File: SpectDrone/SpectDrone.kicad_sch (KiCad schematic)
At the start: 139 parts, among them J1 Conn_02x03_Counter_Clockwise, J1-1 Conn_01x04_Male, J1-2 Conn_01x04_Male, J2 GPS, J3 Barrel_Jack, J3V1-1 Conn_01x01_Male, J3V3 Conn_01x01_Male, J4 BME280, J4V0-1 Conn_01x01_Male, J5 RFShield_OnePiece, J5-1 BNO055-1, J5-2 BNO055-2, J5V3-1 Conn_01x01_Male, J5V3-2 Conn_01x01_Male, J6 Conn_02x16_Counter_Clockwise, J7 Conn_02x16_Counter_Clockwise, Q1 FDN340P, Q2 FDN340P, SW0 SW_Push, SW1 SW_Push, SW10 SW_Push, SW2 SW_Push, SW3 SW_Push, SW4 SW_Push, SW5 SW_Push, SW6 SW_Push, SW7 SW_Push, SW8 SW_Push, SW9 SW_Push, U1 C12666MA, U10 TXS0102DCUR, U11 PCA9306DC, U12 AD799x, U2 C12666MA, U3 MCP112-450E/TO, U4 LM7805_SOT223, U5 MCP112-450E/TO, U6 LM7805_SOT223, U7 Teensy4.0

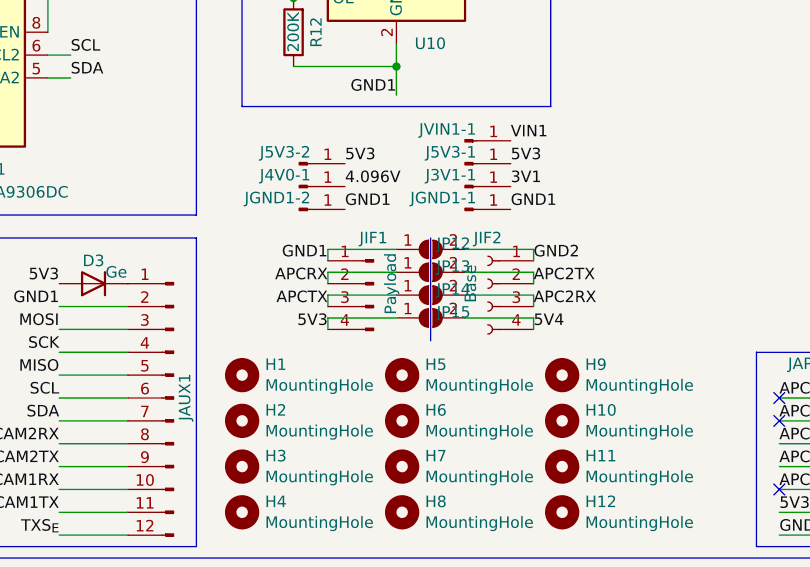
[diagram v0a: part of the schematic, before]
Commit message: SpectDrone Development
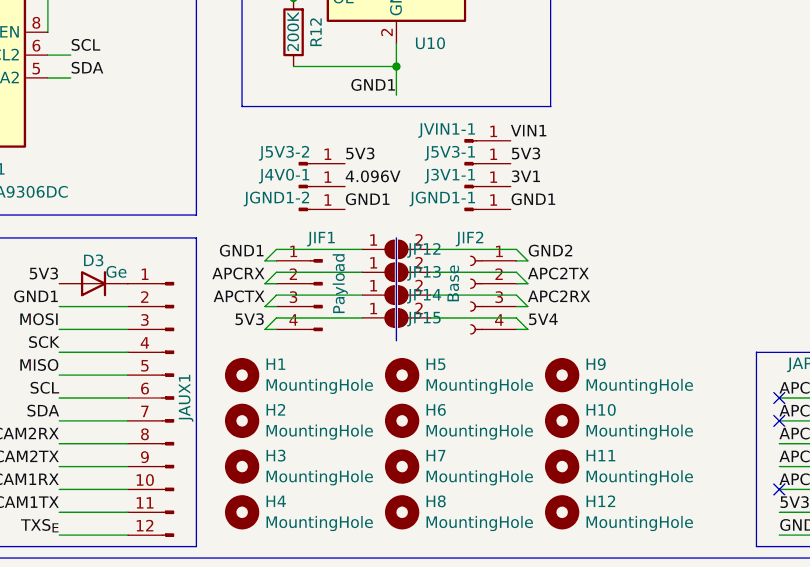
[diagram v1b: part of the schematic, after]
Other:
- moved on the sheet: JIF1, JIF2, JP12, JP13, JP14, JP15
